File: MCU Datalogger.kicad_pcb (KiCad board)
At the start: 2 copper layers, 29 parts, among them J1 Conn_01x04_Pin, J2 Conn_01x09_Pin, J3 Conn_01x04_Pin, J4 Conn_02x03_Odd_Even, U1 24LC1025, U2 DS1337S_, U3 24LC1025, U4 ATMEGA328P-AU, Y1 32.728KHz, Y2 16MHz

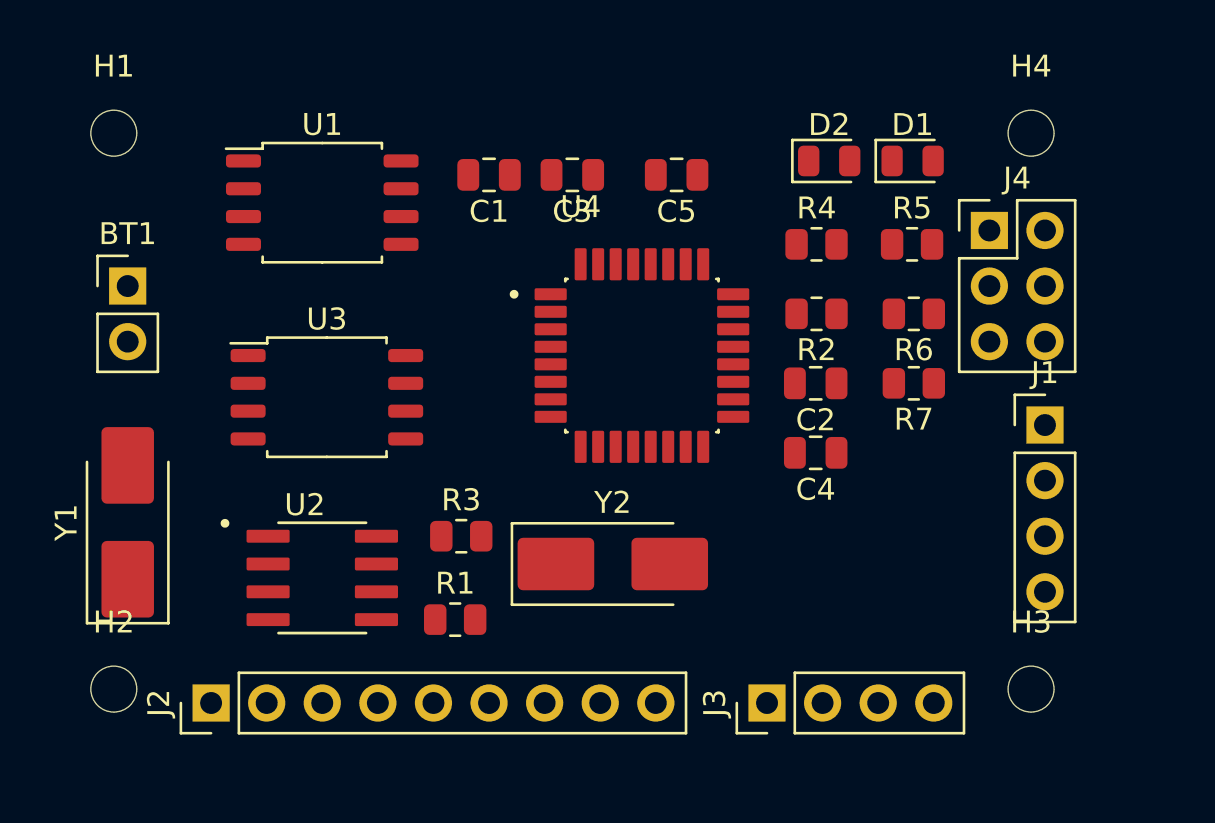
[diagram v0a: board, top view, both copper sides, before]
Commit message: general layout completed ,GND and VCC left
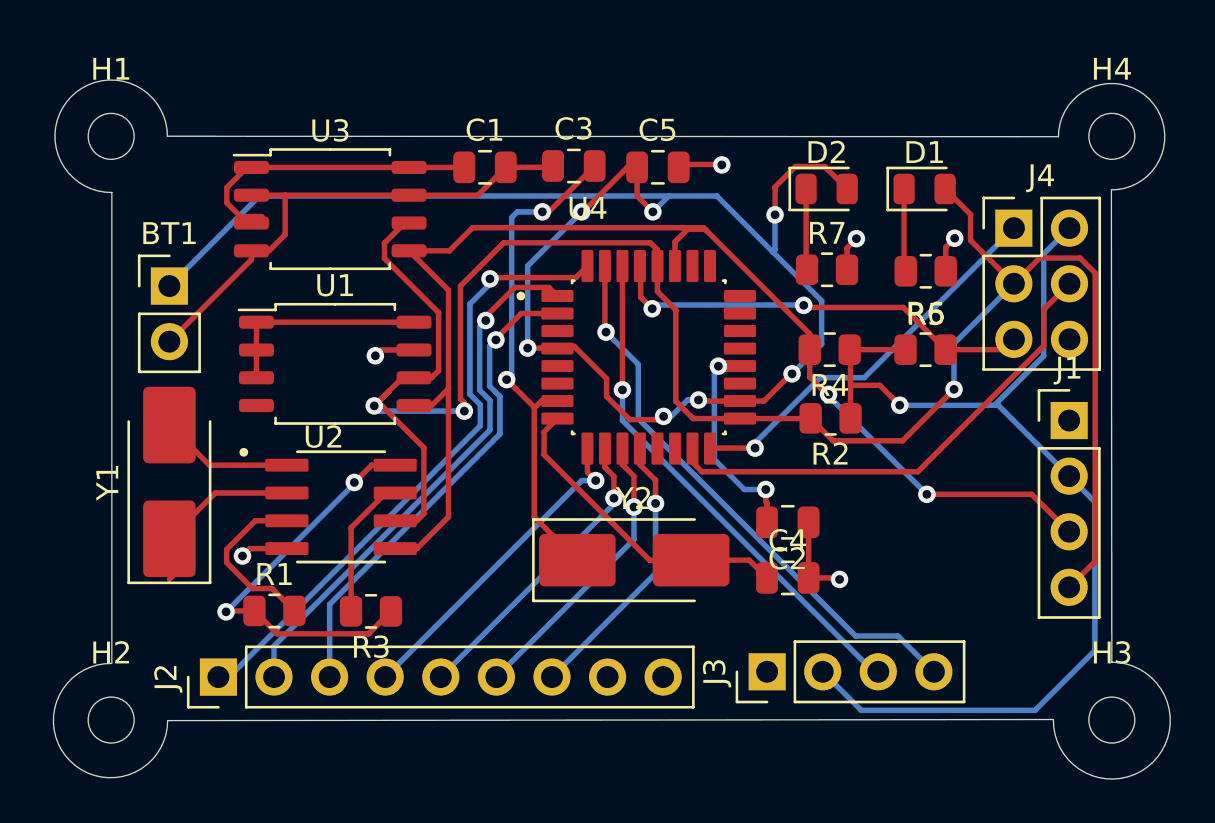
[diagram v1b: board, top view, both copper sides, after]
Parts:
- moved U3 8.60 mm to (139.4, 77.1)
- moved R1 8.27 mm to (136.9, 95.5)
- moved U1 7.39 mm to (139.7, 84.2)
- moved R7 6.53 mm to (162.1, 79.9), turned to 0 degrees
- moved C2 6.48 mm to (160.3, 91.4)
- moved C4 5.86 mm to (160.3, 94.0), turned to 0 degrees
- moved R3 5.37 mm to (141.3, 95.5), turned to 180 degrees
- moved R4 4.85 mm to (162.2, 83.5), turned to 180 degrees
- moved R2 4.82 mm to (162.3, 86.7)
- moved H3 3.95 mm to (175.1, 100.5)
- moved H4 3.69 mm to (175.1, 73.8)
- moved U2 3.36 mm to (139.9, 90.7)
- moved Y1 2.65 mm to (132.1, 89.6)
- moved BT1 1.91 mm to (132.1, 80.6)
- moved R6 1.72 mm to (166.6, 83.5), turned to 0 degrees
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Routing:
- net /VCC: track 0.00 -> 93.3 mm, vias 0 -> 3
- net /SCK: track 0.00 -> 93.1 mm, vias 0 -> 3
- net Net-(BT1-+): track 0.00 -> 73.4 mm, vias 0 -> 7
- net /SDA: track 0.00 -> 58.2 mm, vias 0 -> 2
- net GND: track 0.00 -> 37.7 mm, vias 0 -> 6
- net /D2: track 0.00 -> 28.7 mm, vias 0 -> 1
- net /TX: track 0.00 -> 25.9 mm, vias 0 -> 1
- net /D3: track 0.00 -> 24.9 mm, vias 0 -> 1
- net /RX: track 0.00 -> 23.5 mm, vias 0 -> 1
- net Net-(U4-PB6): track 0.00 -> 23.0 mm, vias 0 -> 2
- net /MOSI: track 0.00 -> 22.6 mm
- net /D4: track 0.00 -> 22.3 mm, vias 0 -> 1
- net /RESET: track 0.00 -> 19.8 mm, vias 0 -> 2
- net /MISO: track 0.00 -> 18.6 mm, vias 0 -> 1
- net /D5: track 0.00 -> 15.0 mm, vias 0 -> 1
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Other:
- board outline added: 51 x 31.9 mm
